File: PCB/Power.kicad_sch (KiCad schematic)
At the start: 10 parts, among them IC2 MC33063ADR

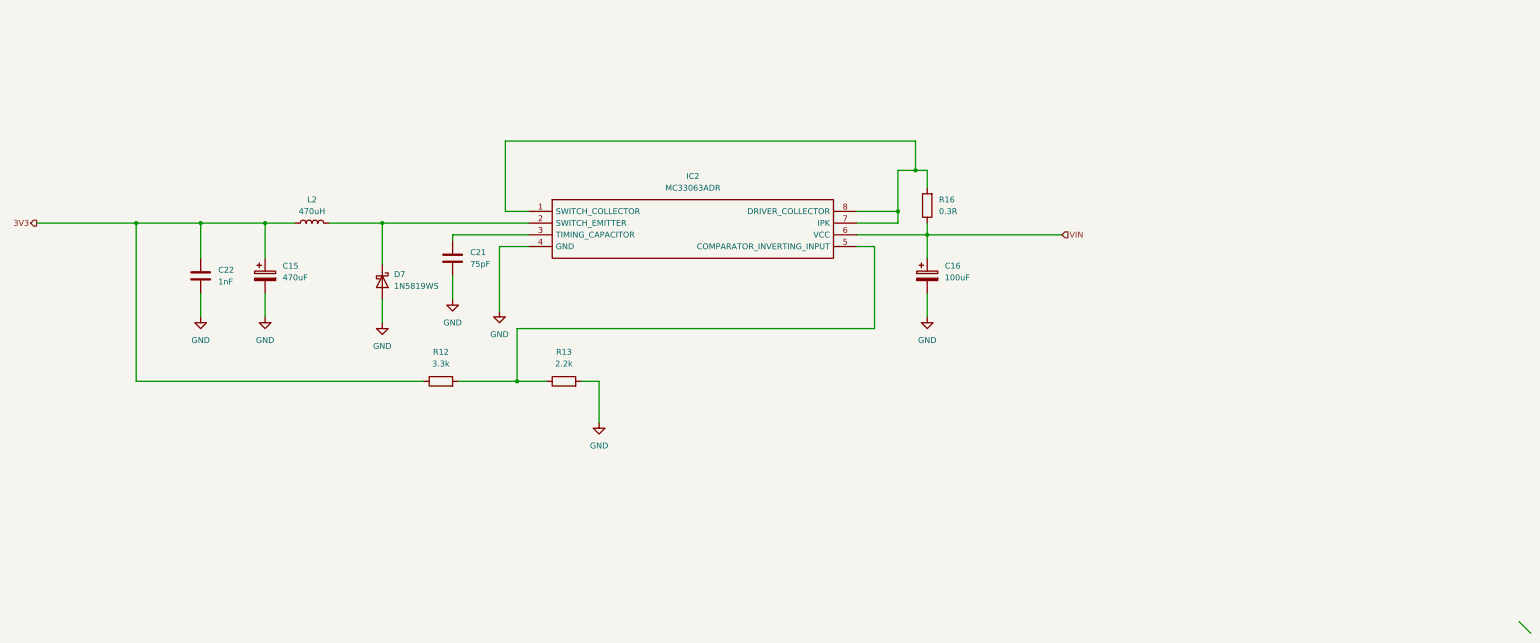
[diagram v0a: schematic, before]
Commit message: Updated PCB
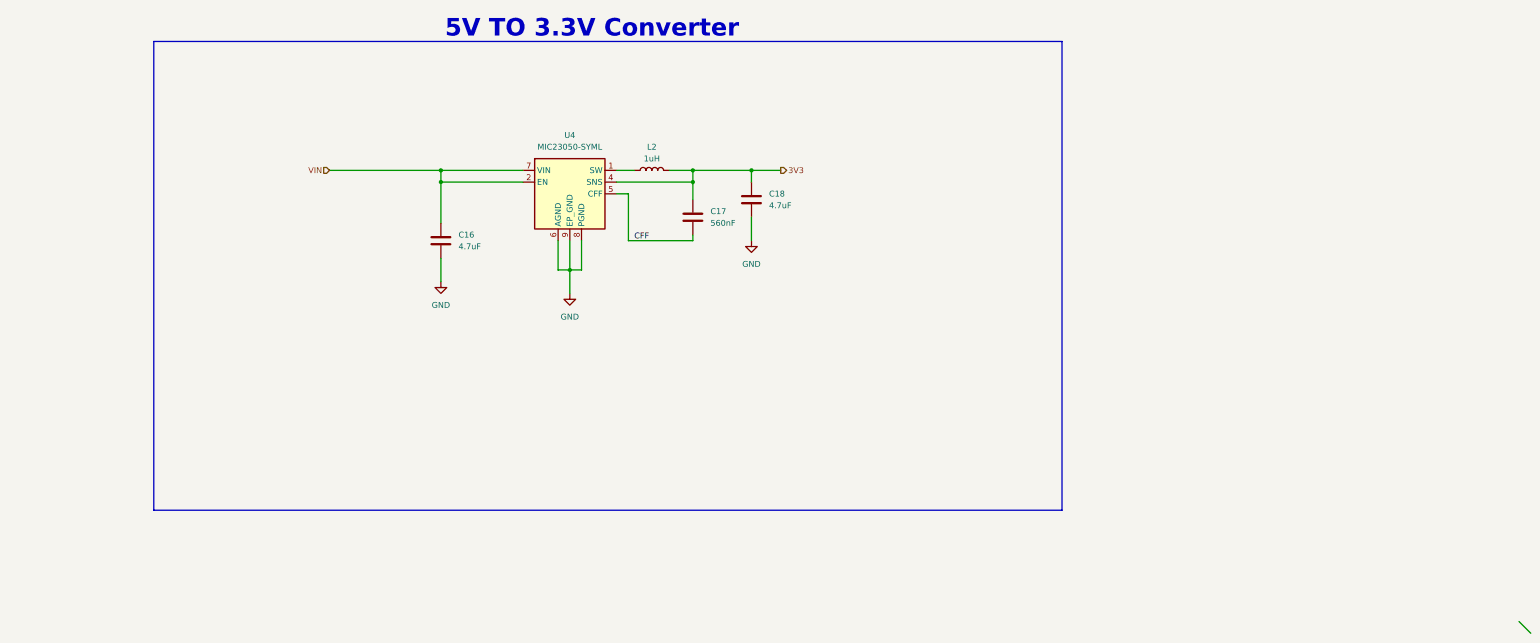
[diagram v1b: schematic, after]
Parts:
- removed C15: 470uF, symbol Device:C_Polarized
- removed C16: 100uF, symbol Device:C_Polarized
- removed C21: 75pF, symbol Device:C
- removed D7: 1N5819WS, Diode_SMD:D_SOD-323, symbol Diode:1N5819WS
- removed IC2: MC33063ADR, Footprints:SOIC127P600X175-8N, symbol IMU_V100:MC33063ADR
- removed R12: 3.3k, symbol Device:R
- removed R13: 2.2k, symbol Device:R
- removed R16: 0.3R, symbol Device:R
- added C17: 560nF, Capacitor_SMD:C_0603_1608Metric, symbol Device:C
- added C18: 4.7uF, Capacitor_SMD:C_0603_1608Metric, symbol Device:C
- added U4: MIC23050-SYML, Package_DFN_QFN:Micrel_MLF-8-1EP_2x2mm_P0.5mm_EP0.6x1.2mm_ThermalVias, symbol Regulator_Switching:MIC23050-SYML
- C16: renamed from C22; value 1nF -> 4.7uF; footprint (none) -> Capacitor_SMD:C_0603_1608Metric
- L2: value 470uH -> 1uH; footprint (none) -> Inductor_SMD:L_0805_2012Metric_Pad1.05x1.20mm_HandSolder
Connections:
- net 3V3: now also L2.2, C17.1, C18.1, U4.4 (SNS); no longer C16.1, L2.1
- net GND: now also C18.2, U4.6 (AGND), U4.8 (PGND), U4.9 (EP_GND)
- net VIN: now also C16.1, U4.2 (EN), U4.7 (VIN)
- new net: L2.1, U4.1 (SW)
- new net CFF: C17.2, U4.5 (CFF)
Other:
- note added: "5V TO 3.3V Converter"
- moved on the sheet: C16
